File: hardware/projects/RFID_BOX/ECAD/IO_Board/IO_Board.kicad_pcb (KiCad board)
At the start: 2 copper layers, 100 x 100 mm, 71 parts, among them J300 J_WAGO_2604-1103, J301 J_WAGO_2604-1103, K300 T92S11D12-24, Q300 2N7002NXAKR, Q301 BSS84AK, Q302 2N7002NXAKR, U300 ISOW7721DFMR, U301 IRM-10-24, U302 MCP39F511A-E/MQ, U306 R-78K5.0-2.0

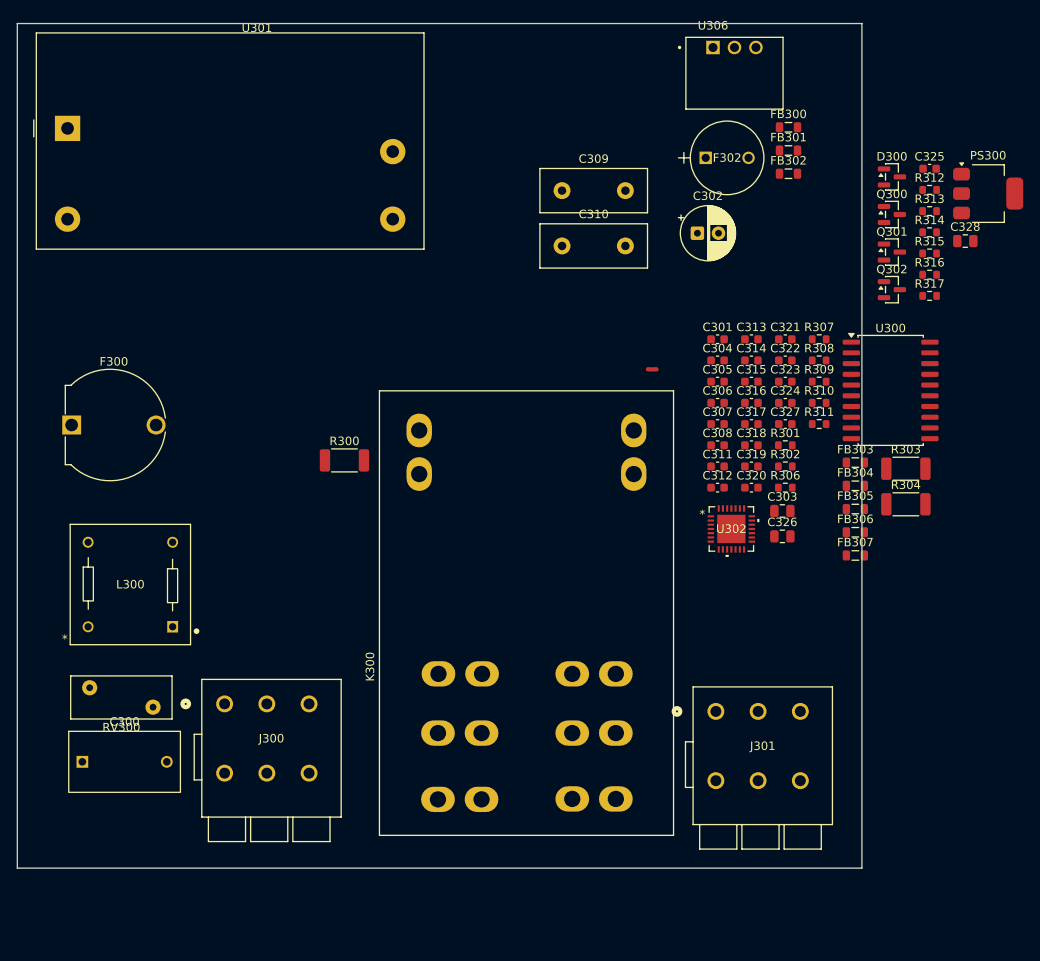
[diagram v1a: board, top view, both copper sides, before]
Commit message: work on layout
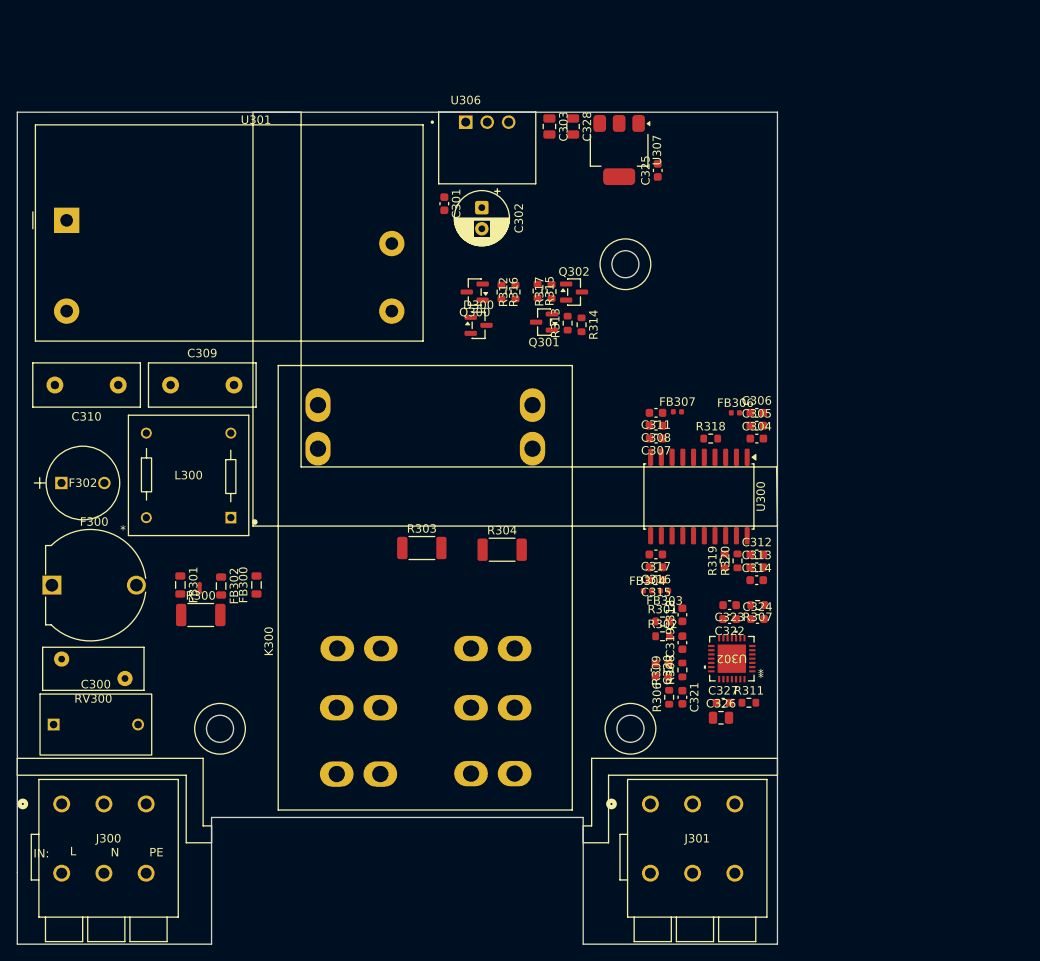
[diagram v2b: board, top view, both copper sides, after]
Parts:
- removed FB305: 330R@100MHz, Inductor_SMD:L_0805_2012Metric
- removed R310: 2R49, Resistor_SMD:R_0603_1608Metric
- added R318: 47k, Resistor_SMD:R_0603_1608Metric, F.Cu at (158.3, 91.7)
- added R319: 0R, Resistor_SMD:R_0603_1608Metric, F.Cu at (159.9, 106.2)
- added R320: 0R, Resistor_SMD:R_0603_1608Metric, F.Cu at (161.5, 106.2)
- FB303, FB304, FB306, FB307: footprint Inductor_SMD:L_0805_2012Metric -> Inductor_SMD:L_0402_1005Metric
- R300: value 2mR CRF2010-FZ-R002ELF -> 2mR
- moved FB301 88.5 mm to (95.5, 109.0), turned to -90 degrees
- moved F302 85.4 mm to (81.4, 96.9)
- moved FB300 83.1 mm to (104.5, 109.0), turned to 90 degrees
- moved FB302 83.0 mm to (100.3, 109.1), turned to -90 degrees
- moved NT300 59.5 mm to (97.8, 109.4), turned to -90 degrees
- moved R303 58.1 mm to (124.1, 104.6)
- moved C310 55.1 mm to (88.2, 85.3), turned to 180 degrees
- moved C303 53.2 mm to (139.2, 54.7), turned to -90 degrees
- moved D300 52.0 mm to (130.8, 78.3)
- moved C309 51.7 mm to (94.3, 85.3)
- moved R316 50.7 mm to (133.5, 74.3), turned to -90 degrees
- moved R312 50.5 mm to (135.2, 74.3), turned to 90 degrees
- moved Q300 50.2 mm to (130.4, 74.3), turned to 180 degrees
- moved C328 48.4 mm to (142.0, 54.7), turned to -90 degrees
- moved R304 48.1 mm to (133.6, 104.8)
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- renumbered PS300 to U307
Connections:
- net /PIN_CTRL_L renamed /PIN_L_CTRL
- net /PIN_CTRL_N renamed /PIN_N_CTRL
- net Earth renamed PIN_PE
- net Net-(F302-Pad2) renamed /PIN_L_CTRL_F
- net Net-(FB300-Pad1) renamed /PIN_L_SENSE
- net Net-(R303-Pad2) renamed /PIN_L_DIV
- net Net-(U302-AVDD) renamed /AVDD
- C307 pad 2: /GND1 -> GND
- C308 pad 2: /GND1 -> GND
- C311 pad 2: /GND1 -> GND
- F300 pad 2: /PIN_FUSED_L -> /PIN_L_FUSED
- FB300 pad 2: /PIN_FUSED_L -> /PIN_L_FUSED
- FB302 pad 2: Net-(FB302-Pad2) -> /PIN_N_SHUNT
- J301 pad 1: Net-(J301-Pin_1) -> /PIN_L_SWITCHED
- J301 pad 2: Net-(J301-Pin_1) -> /PIN_L_SWITCHED
- J301 pad 3: Net-(J301-Pin_3) -> /PIN_N_SWITCHED
- J301 pad 4: Net-(J301-Pin_3) -> /PIN_N_SWITCHED
- K300 pad 2: Net-(J301-Pin_1) -> /PIN_N_SWITCHED
- K300 pad 3: unconnected-(K300-Pad3) -> /PIN_N_nc_1
- K300 pad 4: /PIN_FUSED_L -> /PIN_N_SHUNT
- K300 pad 6: Net-(J301-Pin_3) -> /PIN_L_SWITCHED
- K300 pad 7: unconnected-(K300-Pad7) -> /PIN_L_nc_1
- K300 pad 8: Net-(FB302-Pad2) -> /PIN_L_FUSED
- R300 pad 2: Net-(FB302-Pad2) -> /PIN_N_SHUNT
- R312 pad 2: unconnected-(R312-Pad2) -> /relay_en_LS
- R315 pad 2: unconnected-(R315-Pad2) -> /relay_en_HS
- U300 pad 10: /GND1 -> GND
- U300 pad 5: /VDD -> ISO_EN
- U300 pad 7: /GND1 -> GND
- U302 pad 12: UART_MCP2MCU_ISO -> Net-(U302-UART_TX)
- U302 pad 4: UART_MCU2MCP_ISO -> Net-(U302-UART_RX)
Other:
- board size 100 x 100 mm -> 90 x 98.5 mm
- board text added: "IN:"
- board text added: "L"
- board text added: "N"
- board text added: "PE"
